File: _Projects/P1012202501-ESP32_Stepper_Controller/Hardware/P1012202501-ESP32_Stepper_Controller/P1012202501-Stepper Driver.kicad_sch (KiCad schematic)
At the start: 21 parts, among them CN6 KHS4B-PH-SM4-TB(LF)(SN), CN7 KPTBP04R1-500-04BE, IC6 UDRV8825PWPR, IC7 UTMP36GRTZ-REEL7

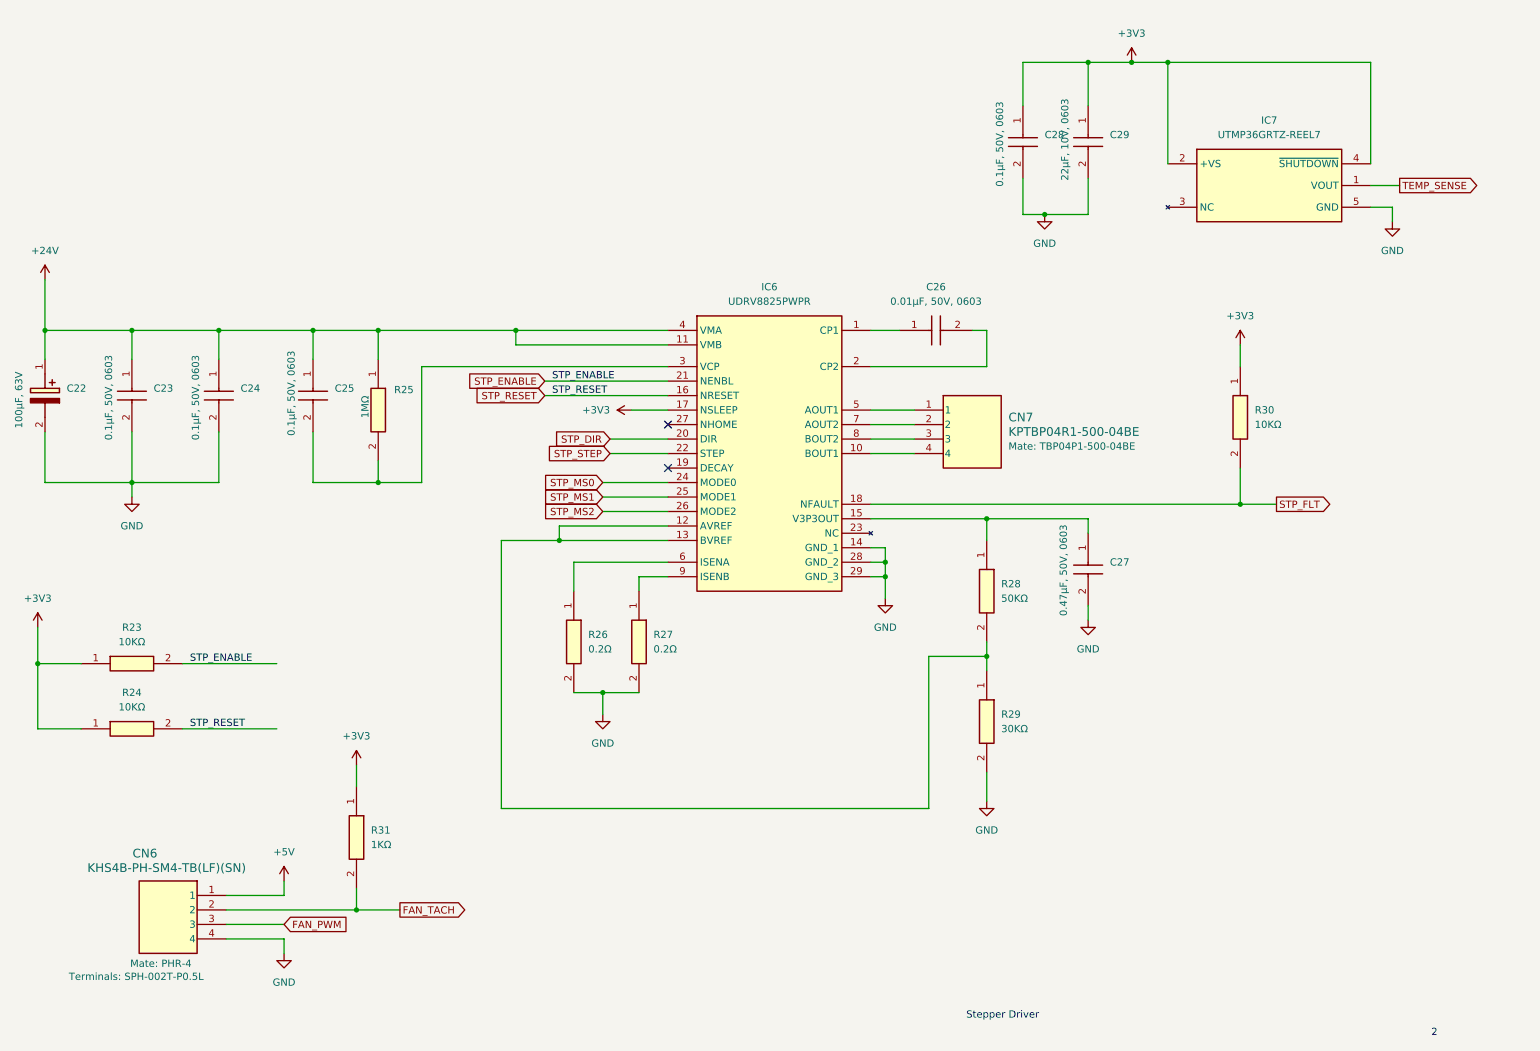
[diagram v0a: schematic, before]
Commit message: Added new items from streams.
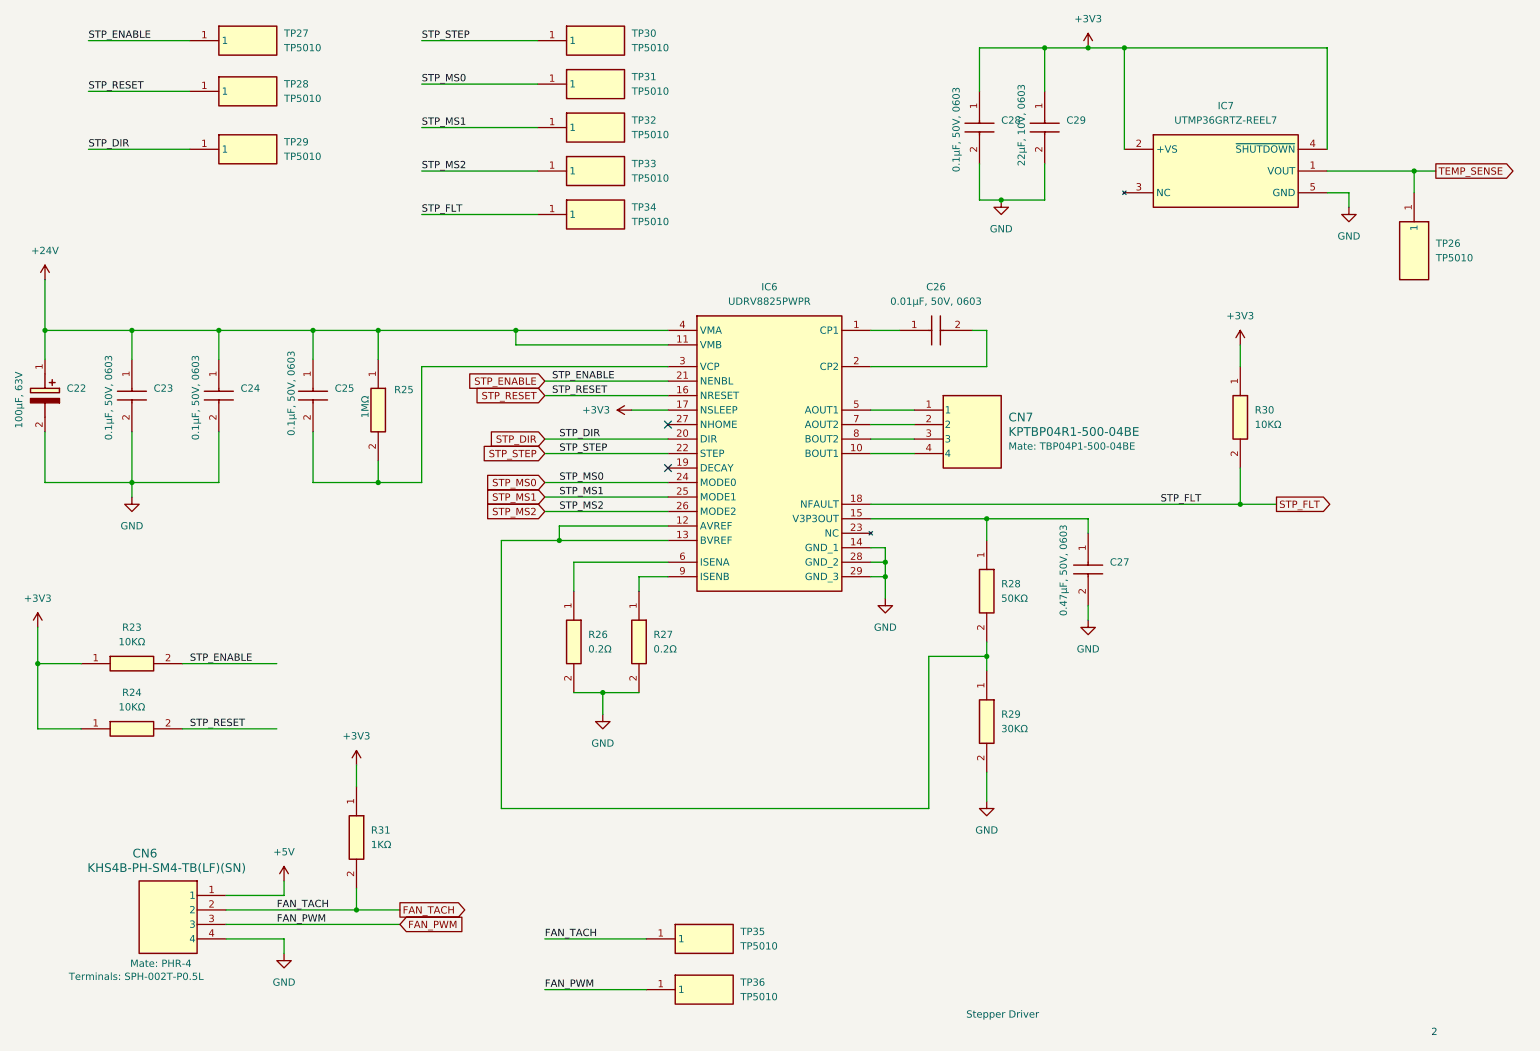
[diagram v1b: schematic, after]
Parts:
- added TP26, TP27, TP28, TP29, TP30, TP31, TP32, TP33, TP34, TP35, TP36: TP5010, CONNECTORS:5010, symbol CONNECTORS:TP5010
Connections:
- net FAN_PWM: now also TP36.1
- net FAN_TACH: now also TP35.1
- net STP_DIR: now also TP29.1
- net STP_ENABLE: now also TP27.1
- net STP_FLT: now also TP34.1
- net STP_MS0: now also TP31.1
- net STP_MS1: now also TP32.1
- net STP_MS2: now also TP33.1
- net STP_RESET: now also TP28.1
- net STP_STEP: now also TP30.1
- net TEMP_SENSE: now also TP26.1
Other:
- moved on the sheet: C28, C29, IC7
